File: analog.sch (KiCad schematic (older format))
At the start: 18 parts, among them J10 Conn_01x04_Male, J11 Conn_01x01_Female, J12 Conn_01x01_Female, J13 Conn_01x01_Female, J14 Conn_02x05_Odd_Even, J8 Conn_01x01_Female, J9 Conn_01x01_Female

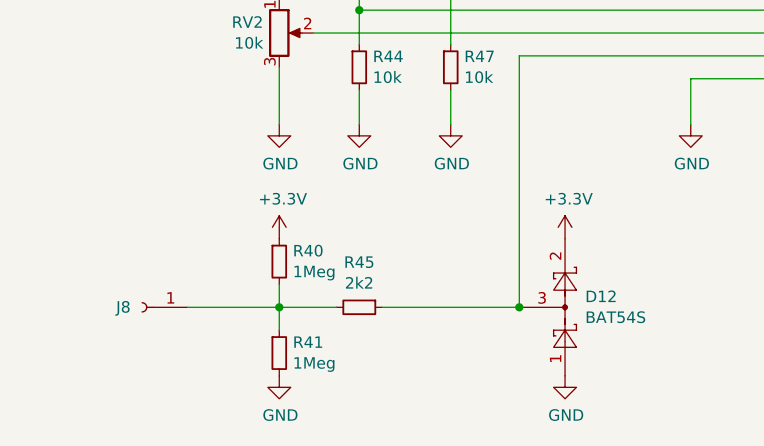
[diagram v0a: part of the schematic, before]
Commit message: Aktuell gefertigte Variante
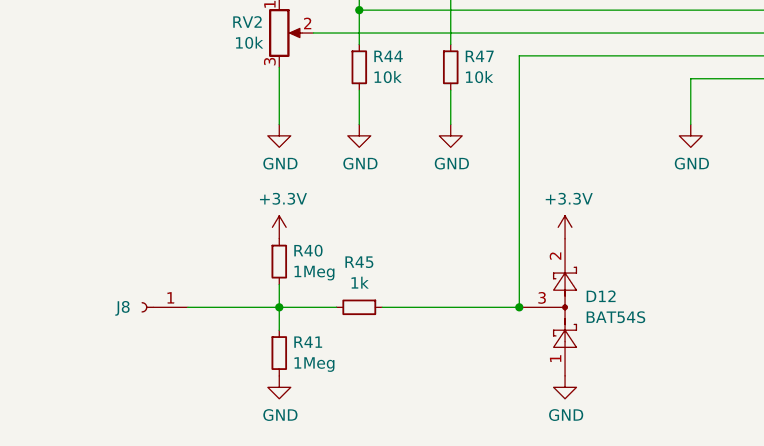
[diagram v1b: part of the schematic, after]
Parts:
- R45: value 2k2 -> 1k
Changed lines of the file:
@@
 P 3000 5850
 F 0 "R45" V 2804 5850 50  0000 C CNN
-F 1 "2k2" V 2895 5850 50  0000 C CNN
+F 1 "1k" V 2895 5850 50  0000 C CNN
 F 2 "Resistor_SMD:R_0603_1608Metric_Pad1.05x0.95mm_HandSolder" H 3000 5850 50  0001 C CNN
 F 3 "~" H 3000 5850 50  0001 C CNN
